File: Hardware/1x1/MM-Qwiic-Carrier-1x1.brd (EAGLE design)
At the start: 80 x 35.6 mm, 87 parts, among them J15 MICROMOD-2222-C, J2 QWIIC_RIGHT_ANGLE, J5 Vertical Qwiic Connector, U1 MCP73831, U5 AP7361C-33FGEUDFN-8

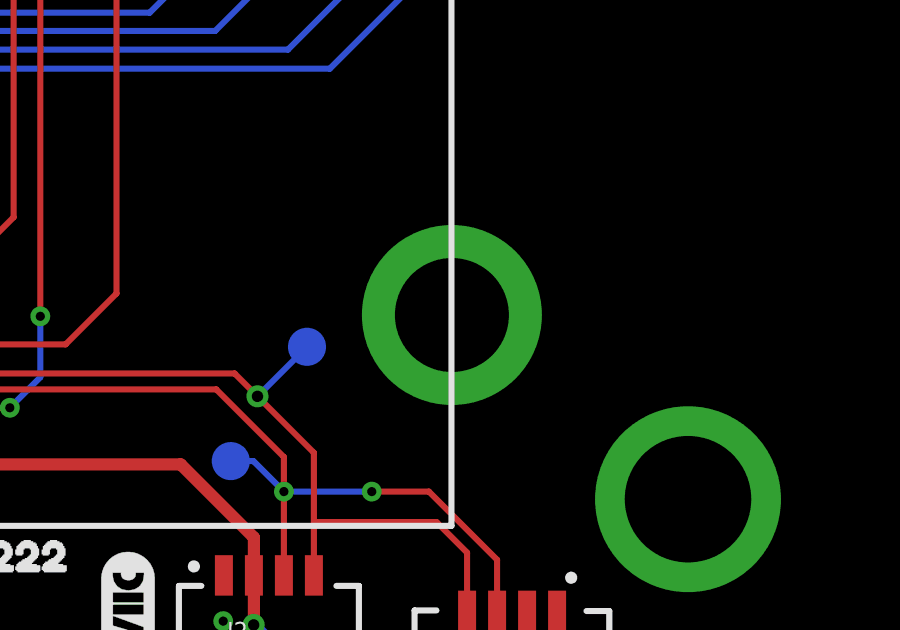
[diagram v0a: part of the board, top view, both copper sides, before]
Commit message: QC Feedback
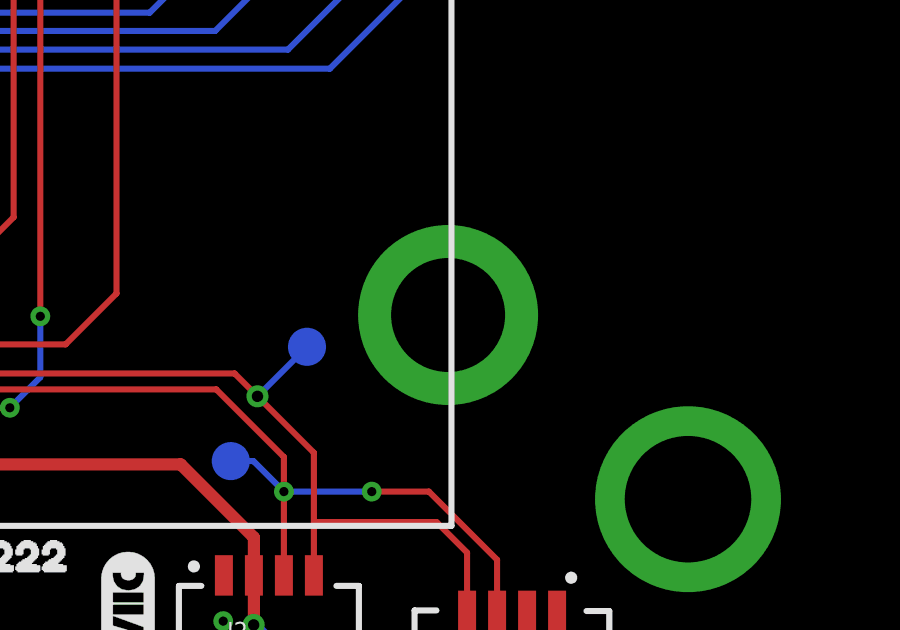
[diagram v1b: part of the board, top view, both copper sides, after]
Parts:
- moved H5 0.13 mm to (44.1, 13.8)
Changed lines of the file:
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@@
 <?xml version="1.0" encoding="utf-8"?>
 <!DOCTYPE eagle SYSTEM "eagle.dtd">
-<eagle version="9.6.2">
+<eagle version="9.5.2">
 <drawing>
 <settings>
-<setting alwaysvectorfont="yes"/>
+<setting alwaysvectorfont="no"/>
 <setting verticaltext="up"/>
 </settings>
@@
 <layer number="45" name="Holes" color="7" fill="1" visible="yes" active="yes"/>
 <layer number="46" name="Milling" color="3" fill="1" visible="no" active="yes"/>
-<layer number="47" name="Measures" color="7" fill="1" visible="no" active="yes"/>
+<layer number="47" name="Measures" color="7" fill="1" visible="yes" active="yes"/>
 <layer number="48" name="Document" color="7" fill="1" visible="no" active="yes"/>
 <layer number="49" name="Reference" color="7" fill="1" visible="no" active="yes"/>
@@
 <wire x1="44.185" y1="6.731" x2="27.94" y2="6.731" width="0.2032" layer="21"/>
 <text x="36.83" y="-21.59" size="1.778" layer="51" font="vector" ratio="15">Priyanka Makin</text>
-<dimension x1="0" y1="35.56" x2="80.01" y2="35.56" x3="40.005" y3="39.37" textsize="1.778" textratio="15" layer="47" unit="inch"/>
-<dimension x1="80.01" y1="35.56" x2="80.01" y2="0" x3="83.82" y3="17.78" textsize="1.778" textratio="15" layer="47" unit="inch"/>
-<text x="43.434" y="39.878" size="1.778" layer="47" font="vector" ratio="15">in</text>
+<dimension x1="0" y1="35.56" x2="80.01" y2="35.56" x3="40.005" y3="45.72" textsize="1.778" textratio="15" layer="47" unit="inch"/>
+<dimension x1="80.01" y1="35.56" x2="80.01" y2="0" x3="91.44" y3="17.78" textsize="1.778" textratio="15" layer="47" unit="inch"/>
+<text x="43.434" y="42.418" size="1.778" layer="47" font="vector" ratio="15">in</text>
+<text x="85.344" y="23.241" size="1.778" layer="47" font="vector" ratio="15" rot="R270">in</text>
+<dimension x1="2.54" y1="33.02" x2="77.47" y2="33.02" x3="40.005" y3="41.91" textsize="1.778" textratio="15" layer="47" unit="inch"/>
+<dimension x1="77.47" y1="33.02" x2="77.47" y2="2.54" x3="87.63" y3="17.78" textsize="1.778" textratio="15" layer="47" unit="inch"/>
+<text x="43.434" y="46.228" size="1.778" layer="47" font="vector" ratio="15">in</text>
+<text x="89.154" y="23.241" size="1.778" layer="47" font="vector" ratio="15" rot="R270">in</text>
+<dimension x1="52.07" y1="27.94" x2="72.39" y2="27.94" x3="62.23" y3="38.1" textsize="1.778" textratio="15" layer="47" unit="inch"/>
+<dimension x1="72.39" y1="27.94" x2="72.39" y2="7.62" x3="83.82" y3="17.78" textsize="1.778" textratio="15" layer="47" unit="inch"/>
 <text x="81.534" y="23.241" size="1.778" layer="47" font="vector" ratio="15" rot="R270">in</text>
-<dimension x1="2.54" y1="33.02" x2="77.47" y2="33.02" x3="40.005" y3="44.45" textsize="1.778" textratio="15" layer="47" unit="inch"/>
-<dimension x1="77.47" y1="33.02" x2="77.47" y2="2.54" x3="88.9" y3="17.78" textsize="1.778" textratio="15" layer="47" unit="inch"/>
-<text x="43.434" y="44.958" size="1.778" layer="47" font="vector" ratio="15">in</text>
-<text x="86.614" y="23.241" size="1.778" layer="47" font="vector" ratio="15" rot="R270">in</text>
+<text x="65.024" y="38.608" size="1.778" layer="47" font="vector" ratio="15">in</text>
 </plain>
 <attributes>
@@
 <element name="LOGO3" library="SparkFun-Aesthetics" package="OSHW-LOGO-M" value="OSHW-LOGOM" x="31.623" y="10.922" smashed="yes" rot="MR0"/>
 <element name="U$55" library="buzzard_labels (9)" package="22229" value="" x="26.962" y="5.72" smashed="yes"/>
-<element name="H5" library="SparkFun-Hardware" package="STAND-OFF-REFLOW-M2.5" value="STAND-OFF-REFLOW2.5MM_TALL" x="44.2" y="13.76" smashed="yes">
-<attribute name="PROD_ID" value="HW-14899" x="44.2" y="13.76" size="1.778" layer="27" font="vector" ratio="15" display="off"/>
+<element name="H5" library="SparkFun-Hardware" package="STAND-OFF-REFLOW-M2.5" value="STAND-OFF-REFLOW2.5MM_TALL" x="44.073" y="13.76" smashed="yes">
+<attribute name="PROD_ID" value="HW-14899" x="44.073" y="13.76" size="1.778" layer="27" font="vector" ratio="15" display="off"/>
 </element>
 <element name="JP4" library="SparkFun-Jumpers" package="SMT-JUMPER_2_NC_TRACE_SILK" package3d_urn="urn:adsk.eagle:package:39281/1" value="3V3 LED" x="15.24" y="33.655" smashed="yes" rot="MR0">
